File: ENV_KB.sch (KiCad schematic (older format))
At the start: 178 parts, among them J1 USB_B_Micro

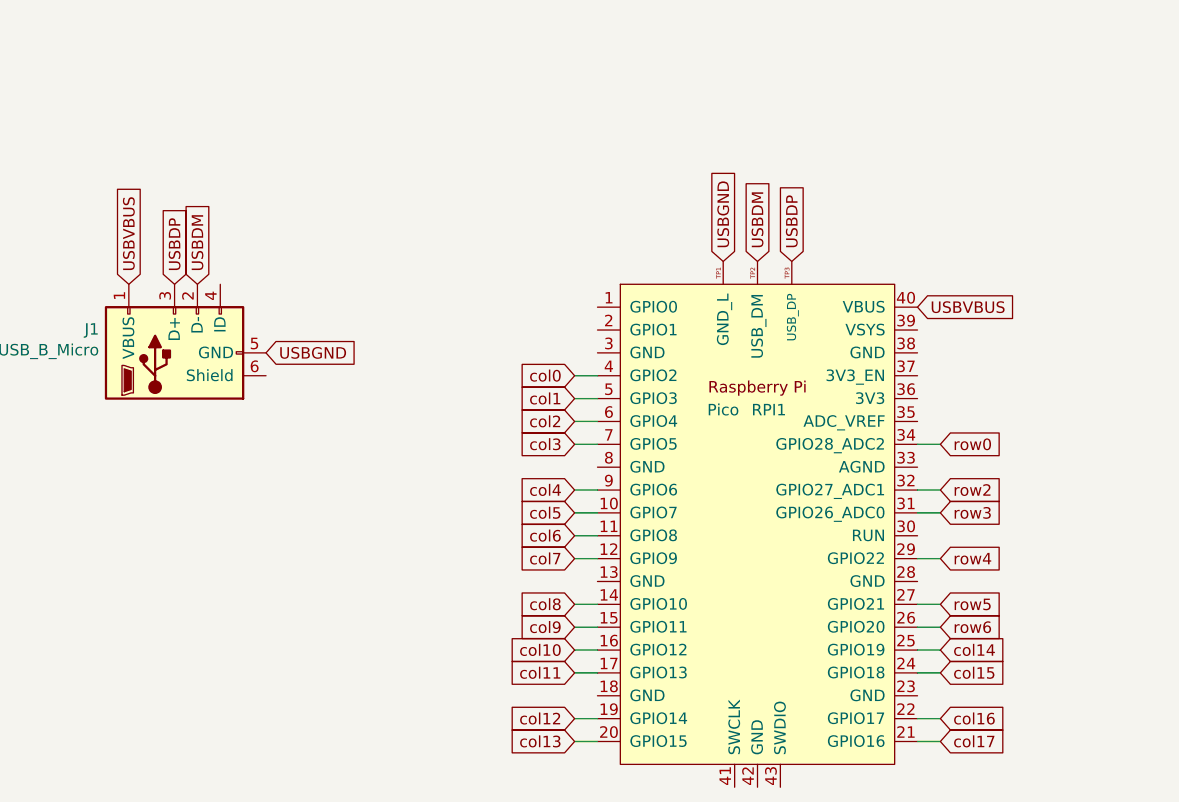
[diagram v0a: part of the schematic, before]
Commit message: This should be Ready.
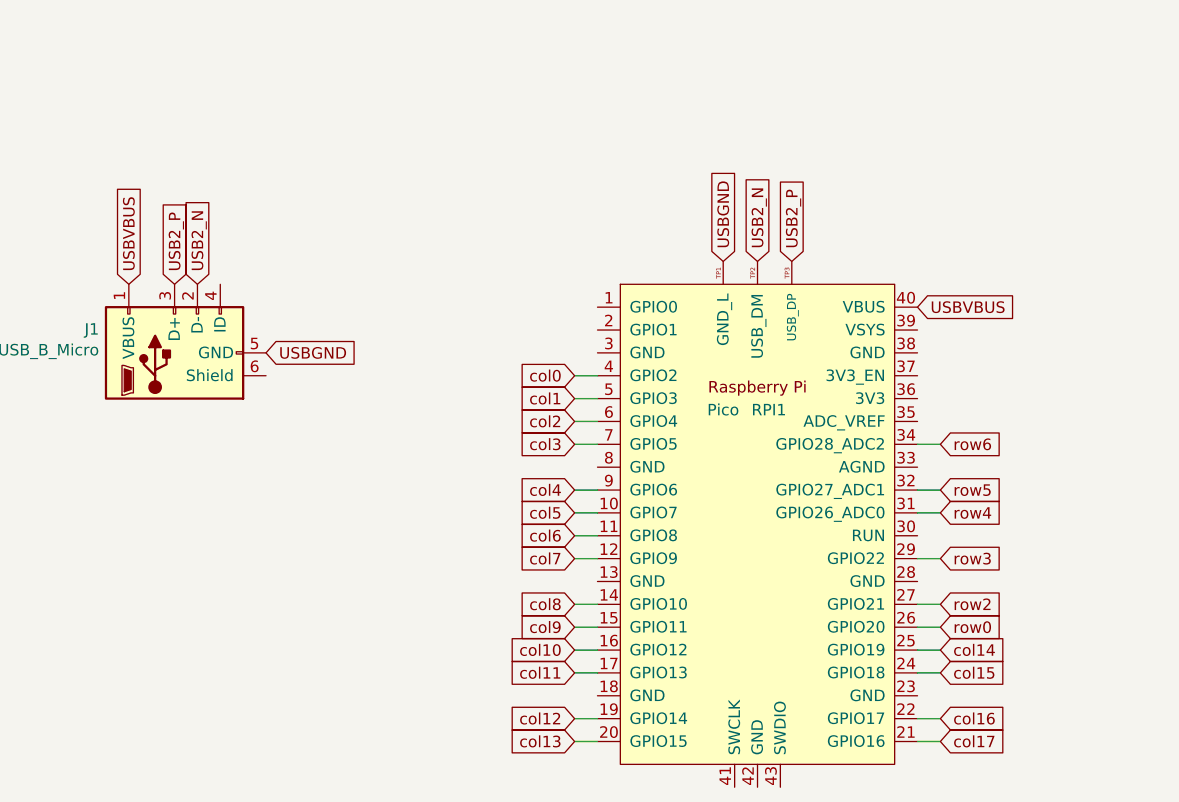
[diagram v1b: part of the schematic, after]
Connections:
- net row0: now also RPI1.26 (GPIO20); no longer RPI1.34 (GPIO28_ADC2)
- net row2: now also RPI1.27 (GPIO21); no longer RPI1.32 (GPIO27_ADC1)
- net row3: now also RPI1.29 (GPIO22); no longer RPI1.31 (GPIO26_ADC0)
- net row4: now also RPI1.31 (GPIO26_ADC0); no longer RPI1.29 (GPIO22)
- net row5: now also RPI1.32 (GPIO27_ADC1); no longer RPI1.27 (GPIO21)
- net row6: now also RPI1.34 (GPIO28_ADC2); no longer RPI1.26 (GPIO20)
- net USBDM renamed USB2_N
- net USBDP renamed USB2_P
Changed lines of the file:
@@
 	0    -1   -1   0
 $EndComp
-Text GLabel 13750 10500 2    50   Input ~ 0
+Text GLabel 13750 9700 2    50   Input ~ 0
 row6
+Text GLabel 13750 9900 2    50   Input ~ 0
+row5
 Text GLabel 13750 10400 2    50   Input ~ 0
-row5
-Text GLabel 13750 9900 2    50   Input ~ 0
 row2
+Text GLabel 13750 10200 2    50   Input ~ 0
+row3
 Text GLabel 13750 10000 2    50   Input ~ 0
-row3
-Text GLabel 13750 10200 2    50   Input ~ 0
 row4
 Text GLabel 13750 10600 2    50   Input ~ 0
@@
 Text GLabel 13750 10700 2    50   Input ~ 0
 col15
-Text GLabel 13750 9700 2    50   Input ~ 0
+Text GLabel 13750 10500 2    50   Input ~ 0
 row0
 Wire Wire Line
@@
 USBGND
 Text GLabel 12950 8900 1    50   Input ~ 0
-USBDM
+USB2_N
 Text GLabel 10500 9000 1    50   Input ~ 0
-USBDM
+USB2_N
 Text GLabel 10400 9000 1    50   Input ~ 0
-USBDP
+USB2_P
 Text GLabel 13100 8900 1    50   Input ~ 0
-USBDP
+USB2_P
 Text GLabel 13650 9100 2    50   Input ~ 0
 USBVBUS
